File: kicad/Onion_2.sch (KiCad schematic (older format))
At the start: 19 parts, among them J3 Conn_01x03, J4 USB_A, SW2 LL3301NF065QG-proy, U5 Omega2-proy

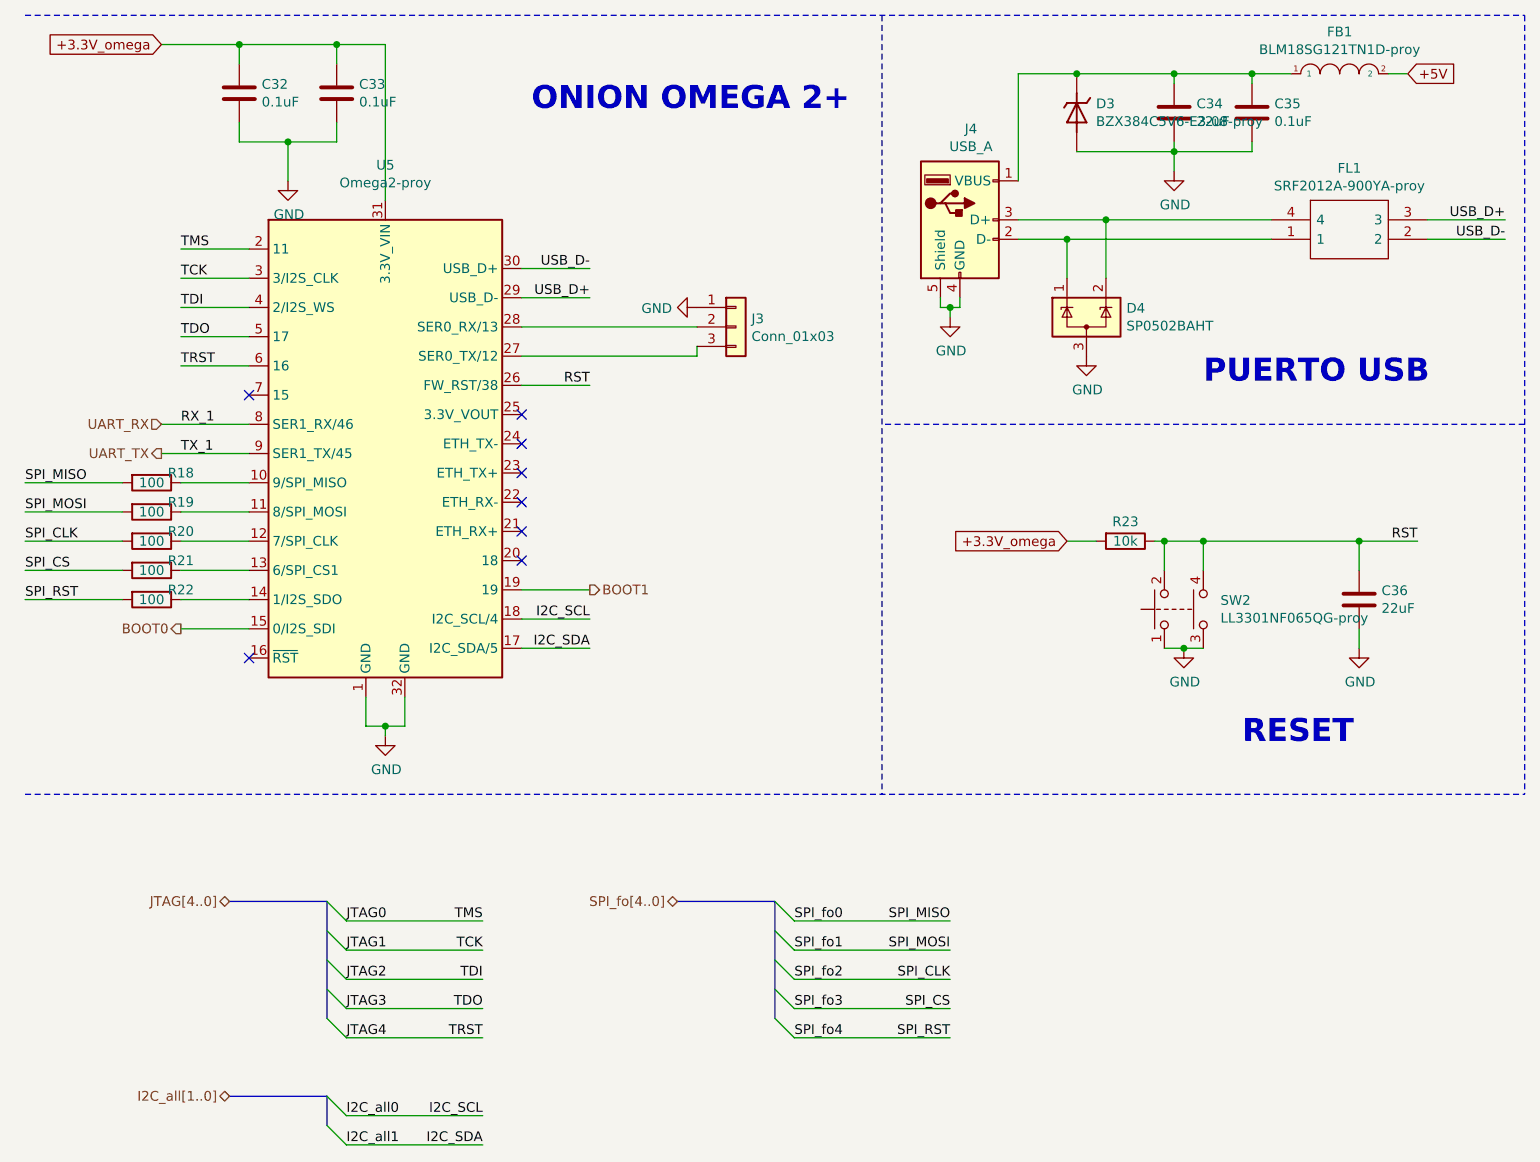
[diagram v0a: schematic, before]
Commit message: Add files via upload
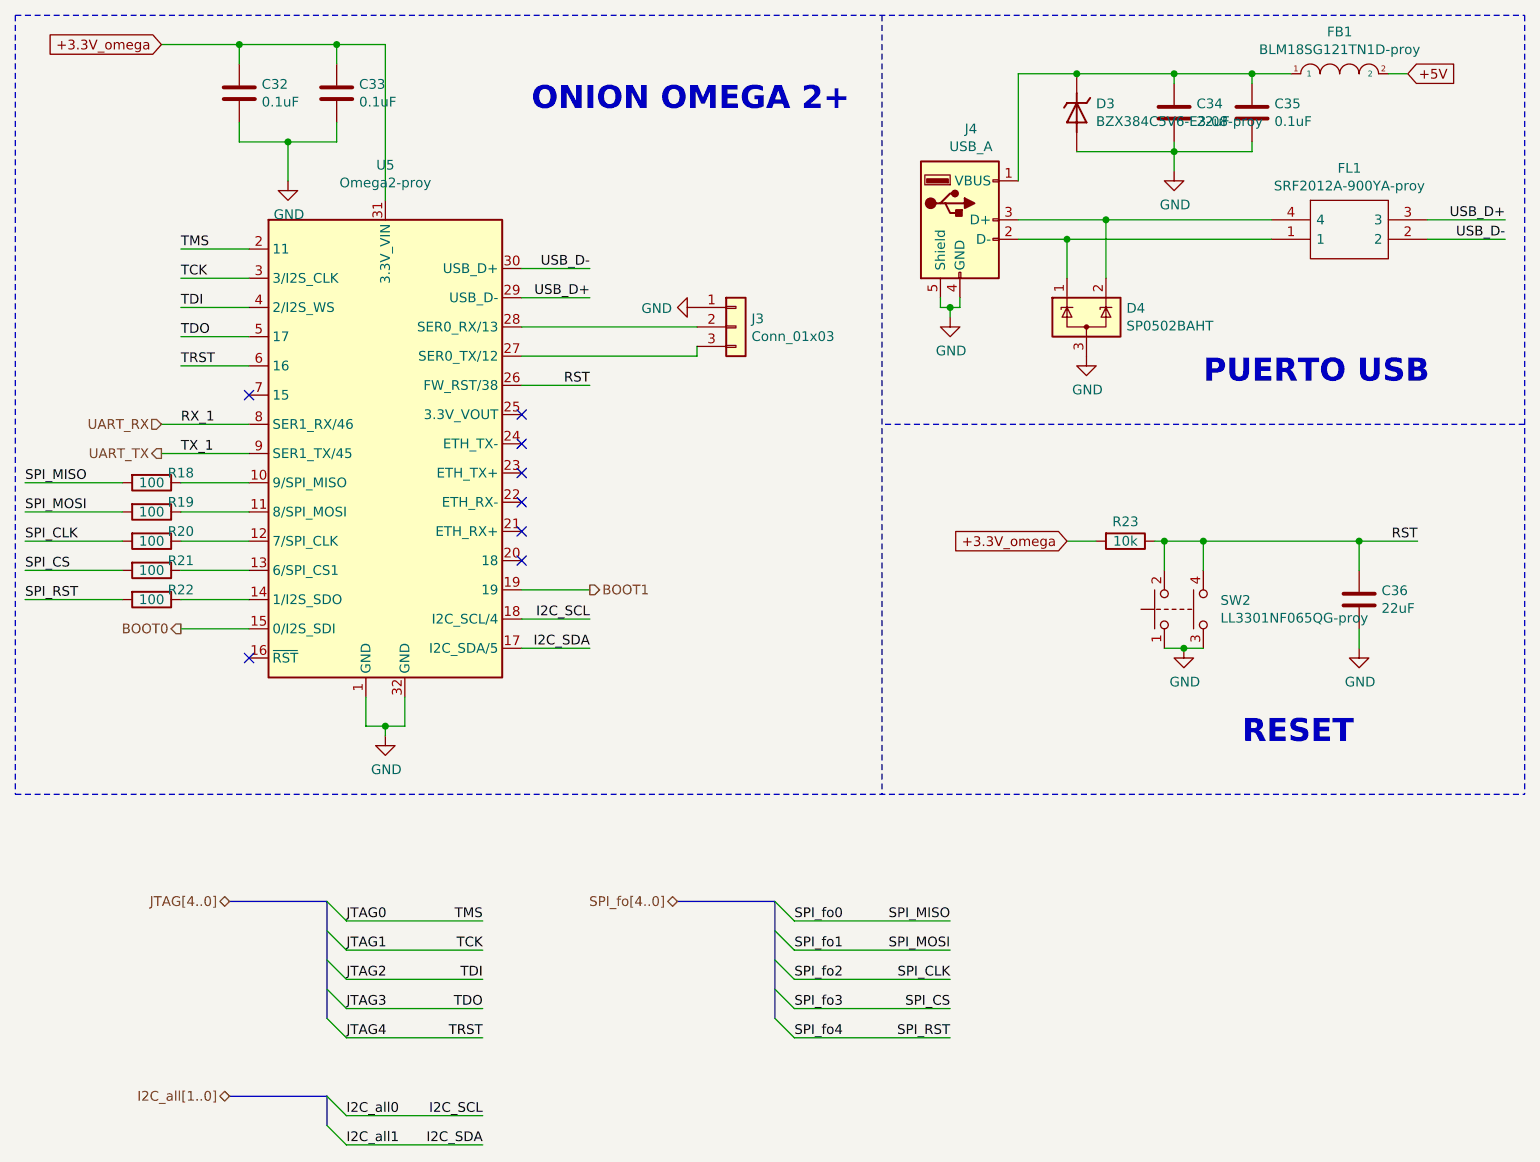
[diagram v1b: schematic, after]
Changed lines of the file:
@@
 Wire Notes Line
 	8300 2650 5000 2650
-Wire Notes Line
-	600  550  8300 550
 Text Notes 6650 2450 0    118  ~ 24
 PUERTO USB\n
-Wire Notes Line
-	600  4550 8300 4550
 Wire Notes Line
 	8300 550  8300 4550
@@
 Wire Wire Line
 	1100 2950 600  2950
+Text Label 5350 5500 2    50   ~ 0
+SPI_CLK
+Text Label 5350 5350 2    50   ~ 0
+SPI_MOSI
+Wire Notes Line
+	550  550  550  4550
+Wire Notes Line
+	550  550  8300 550
+Wire Notes Line
+	550  4550 8300 4550
 Wire Bus Line
 	4450 5100 4450 5700
 Wire Bus Line
 	2150 5100 2150 5700
-Text Label 5350 5500 2    50   ~ 0
-SPI_CLK
-Text Label 5350 5350 2    50   ~ 0
-SPI_MOSI
 $EndSCHEMATC
